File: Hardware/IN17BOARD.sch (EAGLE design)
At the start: 53 parts, among them IC1 IC_74141-DIP-16, J1 AVR_SPI_PRG_62X3_LOCK, Q1 MPSA42, Q2 MPSA92, Q3 MPSA42, Q4 MPSA92, Q5 MPSA42, Q6 MPSA92, Q7 MPSA42, Q8 MPSA92

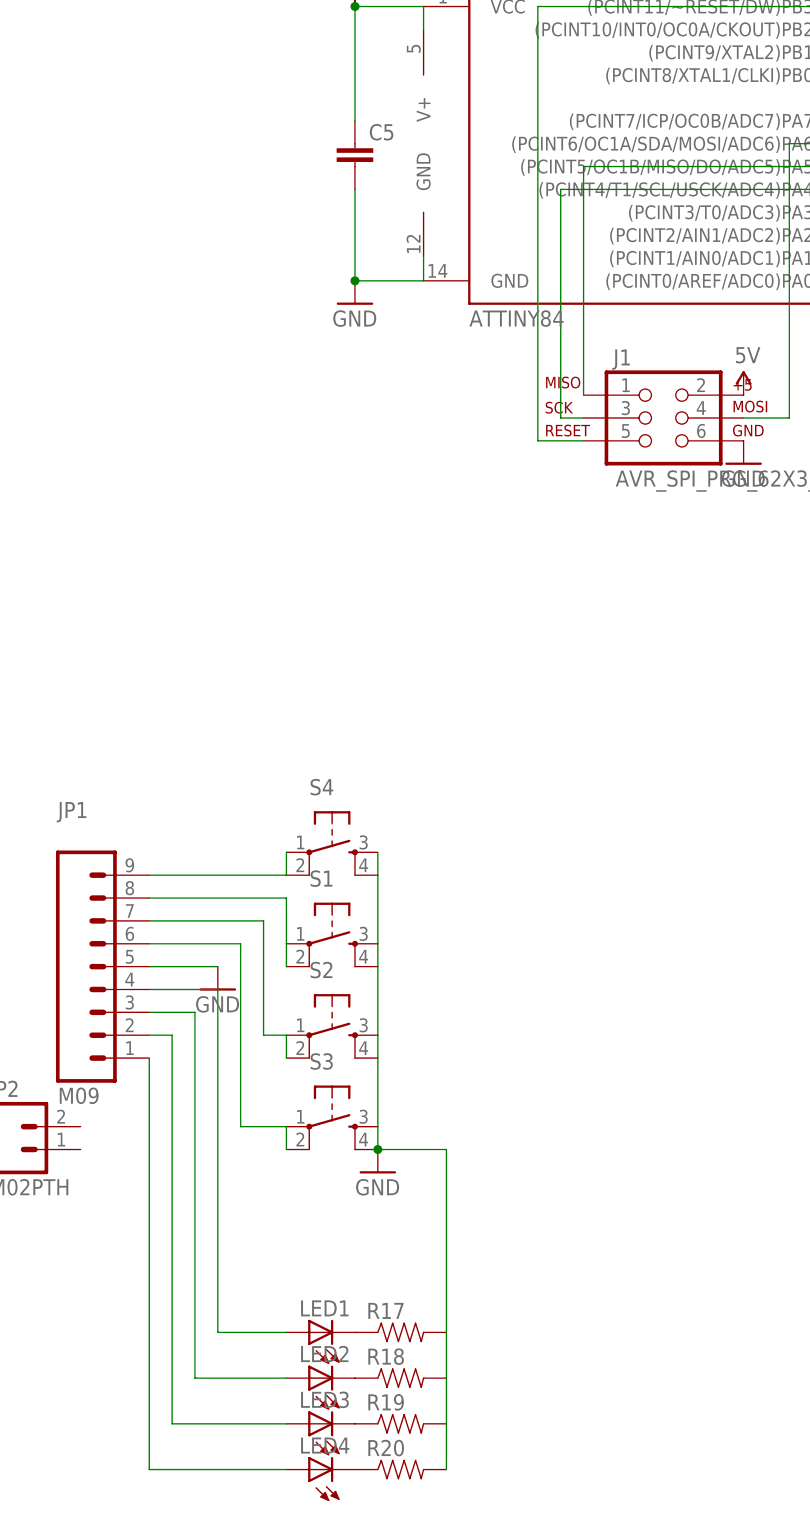
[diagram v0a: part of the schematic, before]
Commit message: Add value and main sketch
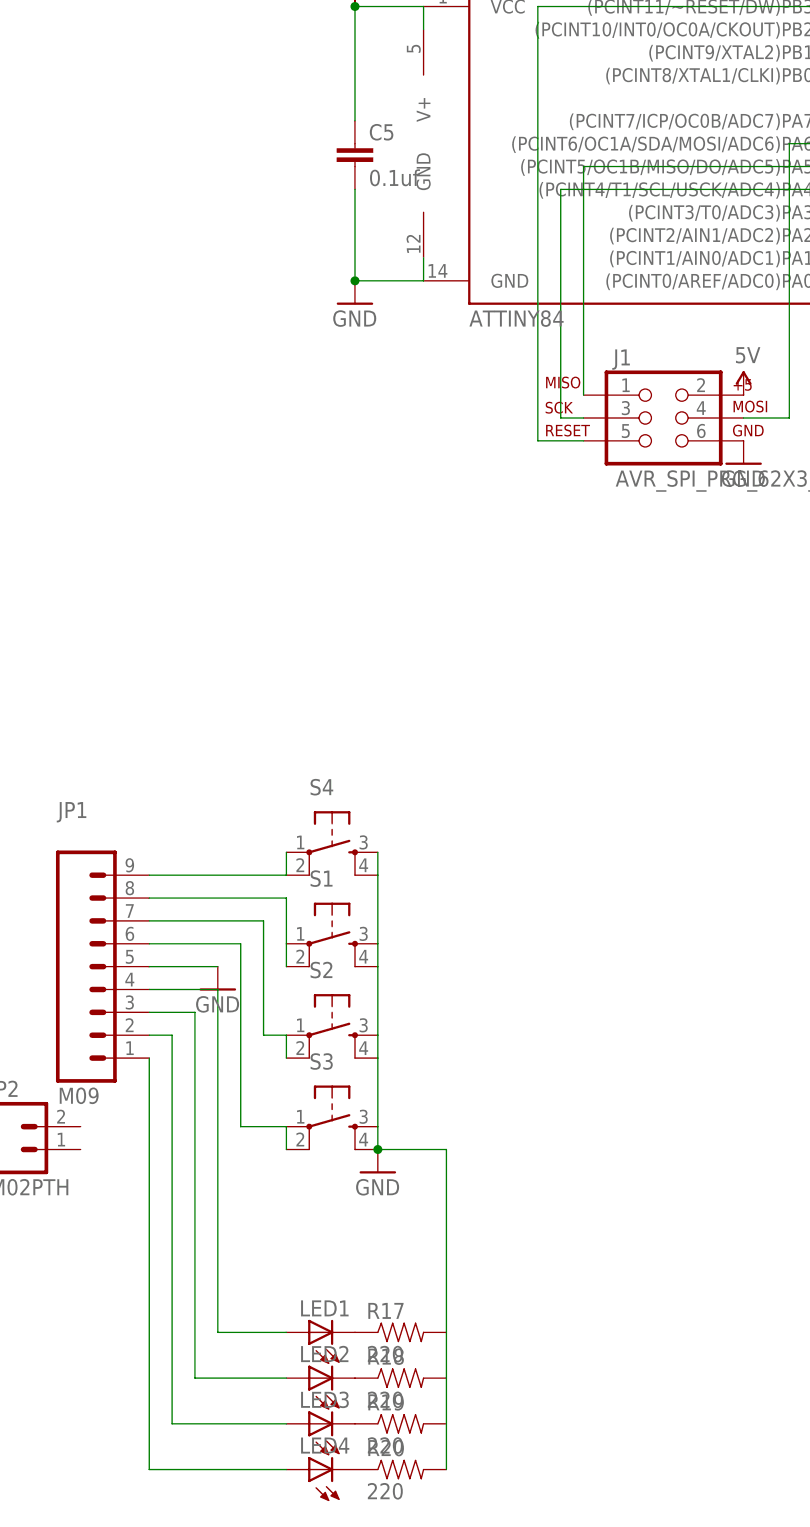
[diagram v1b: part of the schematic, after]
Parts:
- C5: value (none) -> 0.1uf
- R17, R18, R19, R20: value (none) -> 220
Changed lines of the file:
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@@
 <part name="H1" library="holes" deviceset="MOUNT-HOLE" device="3.0"/>
 <part name="H2" library="holes" deviceset="MOUNT-HOLE" device="3.0"/>
-<part name="C5" library="SparkFun-Capacitors" deviceset="CAP" device="0805"/>
+<part name="C5" library="SparkFun-Capacitors" deviceset="CAP" device="0805" value="0.1uf"/>
 <part name="SUPPLY2" library="SparkFun-Aesthetics" deviceset="5V" device=""/>
 <part name="GND5" library="SparkFun-Aesthetics" deviceset="GND" device=""/>
@@
 <part name="LED3" library="SparkFun-LED" deviceset="LED" device="0603"/>
 <part name="LED4" library="SparkFun-LED" deviceset="LED" device="0603"/>
-<part name="R17" library="SparkFun-Resistors" deviceset="RESISTOR" device="0603-RES"/>
-<part name="R18" library="SparkFun-Resistors" deviceset="RESISTOR" device="0603-RES"/>
-<part name="R19" library="SparkFun-Resistors" deviceset="RESISTOR" device="0603-RES"/>
-<part name="R20" library="SparkFun-Resistors" deviceset="RESISTOR" device="0603-RES"/>
+<part name="R17" library="SparkFun-Resistors" deviceset="RESISTOR" device="0603-RES" value="220"/>
+<part name="R18" library="SparkFun-Resistors" deviceset="RESISTOR" device="0603-RES" value="220"/>
+<part name="R19" library="SparkFun-Resistors" deviceset="RESISTOR" device="0603-RES" value="220"/>
+<part name="R20" library="SparkFun-Resistors" deviceset="RESISTOR" device="0603-RES" value="220"/>
 <part name="JP1" library="SparkFun-Connectors" deviceset="M09" device=""/>
 <part name="Q2" library="SparkFun-DiscreteSemi" deviceset="TRANSISTOR_PNP" device="MMBT3906" value="MPSA92"/>
